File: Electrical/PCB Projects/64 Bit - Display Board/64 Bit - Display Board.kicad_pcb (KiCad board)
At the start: 4 copper layers, 200 x 75.1 mm, 60 parts, among them J1 Conn_01x03, J2 Conn_01x03, P1 610110249121, P2 610110249121, P3 610110249121, T1 IN-12A, T10 IN-12A, T2 IN-12A, T5 IN-12A, T6 IN-12A, T9 IN-12A, U1 TPIC6B595, U2 TPIC6B595, U3 TPIC6B595, U4 TPIC6B595, U5 TPIC6B595, U6 TPIC6B595, U7 TPIC6B595, U8 TPIC6B595

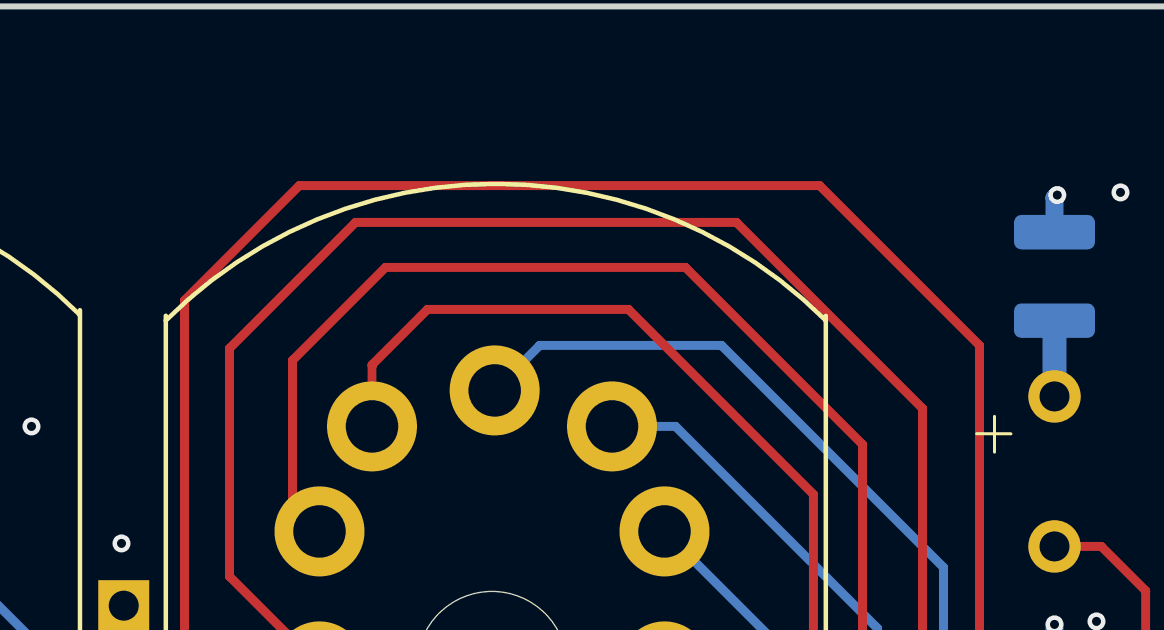
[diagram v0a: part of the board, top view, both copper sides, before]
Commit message: slight changes
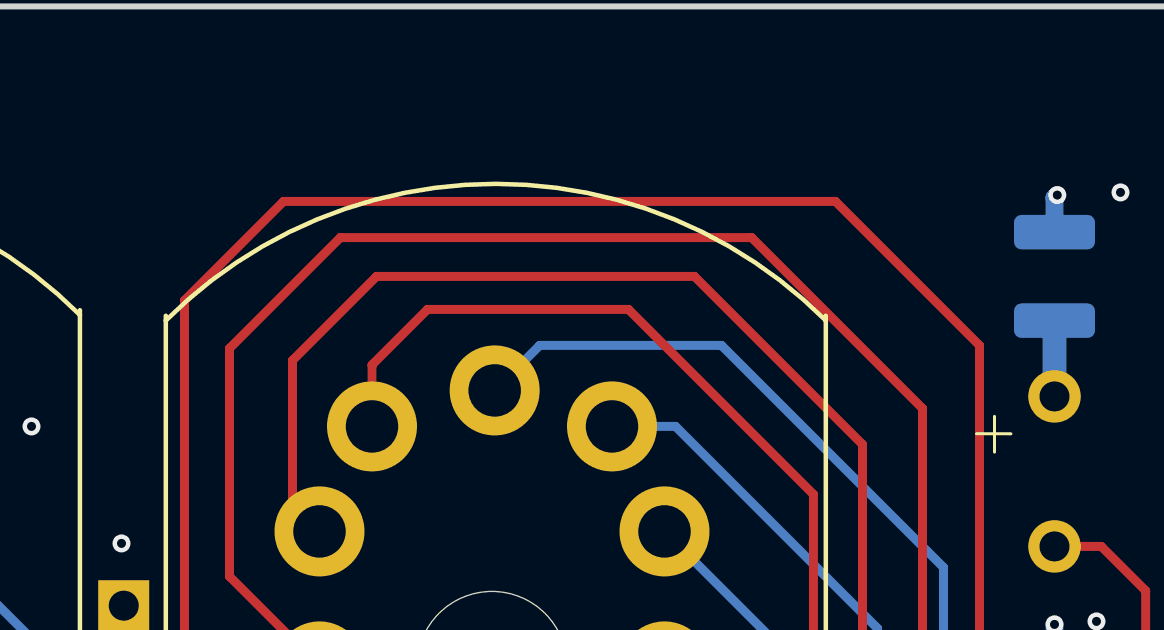
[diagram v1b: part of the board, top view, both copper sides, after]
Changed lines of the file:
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@@
+	)
+	(segment
+		(start 106.5 56.5)
+		(end 95.9 56.5)
+		(width 0.3)
+		(layer "F.Cu")
+		(net 72)
+	)
+	(segment
+		(start 93.1 59.3)
+		(end 93.1 64.1)
+		(width 0.3)
+		(layer "F.Cu")
+		(net 72)
+	)
+	(segment
+		(start 117.5 96.1)
+		(end 112.1 90.7)
+		(width 0.3)
+		(layer "F.Cu")
+		(net 72)
+	)
+	(segment
+		(start 112.1 62.1)
+		(end 106.5 56.5)
+		(width 0.3)
+		(layer "F.Cu")
+		(net 72)
+	)
+	(segment
+		(start 112.1 90.7)
+		(end 112.1 62.1)
+		(width 0.3)
+		(layer "F.Cu")
+		(net 72)
+	)
+	(segment
+		(start 121.567267 92.442808)
+		(end 121.567267 92.432733)
+		(width 0.3)
+		(layer "F.Cu")
+		(net 72)
 	)
 	(segment
@@
 	)
 	(segment
-		(start 117.5 96.1)
-		(end 112.1 90.7)
-		(width 0.3)
-		(layer "F.Cu")
-		(net 72)
-	)
-	(segment
-		(start 93.1 59.3)
-		(end 93.1 64.1)
-		(width 0.3)
-		(layer "F.Cu")
-		(net 72)
-	)
-	(segment
-		(start 112.1 62.1)
-		(end 106.2 56.2)
-		(width 0.3)
-		(layer "F.Cu")
-		(net 72)
-	)
-	(segment
-		(start 96.2 56.2)
+		(start 95.9 56.5)
 		(end 93.1 59.3)
-		(width 0.3)
-		(layer "F.Cu")
-		(net 72)
-	)
-	(segment
-		(start 121.567267 92.442808)
-		(end 121.567267 92.432733)
-		(width 0.3)
-		(layer "F.Cu")
-		(net 72)
-	)
-	(segment
-		(start 112.1 90.7)
-		(end 112.1 62.1)
-		(width 0.3)
-		(layer "F.Cu")
-		(net 72)
-	)
-	(segment
-		(start 106.2 56.2)
-		(end 96.2 56.2)
 		(width 0.3)
 		(layer "F.Cu")
@@
 	)
 	(segment
+		(start 91 58.9)
+		(end 91 66.5)
+		(width 0.3)
+		(layer "F.Cu")
+		(net 79)
+	)
+	(segment
+		(start 114.1 90.5)
+		(end 114.1 60.9)
+		(width 0.3)
+		(layer "F.Cu")
+		(net 79)
+	)
+	(segment
 		(start 91 66.5)
 		(end 94 69.5)
@@
 	)
 	(segment
+		(start 108.40569 55.20569)
+		(end 94.69431 55.20569)
+		(width 0.3)
+		(layer "F.Cu")
+		(net 79)
+	)
+	(segment
+		(start 114.1 60.9)
+		(end 108.40569 55.20569)
+		(width 0.3)
+		(layer "F.Cu")
+		(net 79)
+	)
+	(segment
 		(start 119.4 95.8)
 		(end 114.1 90.5)
@@
 	)
 	(segment
-		(start 107.9 54.7)
-		(end 95.2 54.7)
-		(width 0.3)
-		(layer "F.Cu")
-		(net 79)
-	)
-	(segment
-		(start 95.2 54.7)
-		(end 91 58.9)
-		(width 0.3)
-		(layer "F.Cu")
-		(net 79)
-	)
-	(segment
-		(start 91 58.9)
-		(end 91 66.5)
-		(width 0.3)
-		(layer "F.Cu")
-		(net 79)
-	)
-	(segment
 		(start 122.559167 93.340833)
 		(end 124 91.9)
@@
 	)
 	(segment
-		(start 114.1 90.5)
-		(end 114.1 60.9)
-		(width 0.3)
-		(layer "F.Cu")
-		(net 79)
-	)
-	(segment
-		(start 114.1 60.9)
-		(end 107.9 54.7)
+		(start 94.69431 55.20569)
+		(end 91 58.9)
 		(width 0.3)
 		(layer "F.Cu")
@@
 	)
 	(segment
+		(start 116 90.2)
+		(end 116 58.8)
+		(width 0.3)
+		(layer "F.Cu")
+		(net 80)
+	)
+	(segment
 		(start 120.811072 95.011072)
 		(end 116 90.2)
@@
 	)
 	(segment
-		(start 93.328049 53.471951)
+		(start 116 58.8)
+		(end 111.2 54)
+		(width 0.3)
+		(layer "F.Cu")
+		(net 80)
+	)
+	(segment
+		(start 111.2 54)
+		(end 92.8 54)
+		(width 0.3)
+		(layer "F.Cu")
+		(net 80)
+	)
+	(segment
+		(start 92.8 54)
 		(end 89.5 57.3)
 		(width 0.3)
@@
 	)
 	(segment
-		(start 110.671951 53.471951)
-		(end 93.328049 53.471951)
+		(start 89.5 69.5)
+		(end 94 74)
+		(width 0.3)
+		(layer "F.Cu")
+		(net 80)
+	)
+	(segment
+		(start 89.5 57.3)
+		(end 89.5 69.5)
 		(width 0.3)
 		(layer "F.Cu")
@@
 	)
 	(segment
-		(start 89.5 69.5)
-		(end 94 74)
-		(width 0.3)
-		(layer "F.Cu")
-		(net 80)
-	)
-	(segment
 		(start 122.591105 95.011072)
 		(end 120.811072 95.011072)
-		(width 0.3)
-		(layer "F.Cu")
-		(net 80)
-	)
-	(segment
-		(start 89.5 57.3)
-		(end 89.5 69.5)
-		(width 0.3)
-		(layer "F.Cu")
-		(net 80)
-	)
-	(segment
-		(start 116 90.2)
-		(end 116 58.8)
-		(width 0.3)
-		(layer "F.Cu")
-		(net 80)
-	)
-	(segment
-		(start 116 58.8)
-		(end 110.671951 53.471951)
 		(width 0.3)
 		(layer "F.Cu")
@@
 		(net 2)
 		(net_name "GND")
-		(layers "F.Cu" "B.Cu")
+		(layers "F.Cu" "B.Cu" "In1.Cu")
 		(hatch edge 0.5)
 		(priority 1)
@@
 		(net 2)
 		(net_name "GND")
-		(layers "F.Cu" "B.Cu")
+		(layers "F.Cu" "B.Cu" "In1.Cu")
 		(hatch edge 0.5)
 		(priority 1)
@@
 		(net 2)
 		(net_name "GND")
-		(layers "F.Cu" "B.Cu")
+		(layers "F.Cu" "B.Cu" "In1.Cu")
 		(hatch edge 0.5)
 		(priority 1)
@@
 		(net 2)
 		(net_name "GND")
-		(layers "F.Cu" "B.Cu")
+		(layers "F.Cu" "B.Cu" "In1.Cu")
 		(hatch edge 0.5)
 		(priority 1)
@@
 		(net 2)
 		(net_name "GND")
-		(layers "F.Cu" "B.Cu")
+		(layers "F.Cu" "B.Cu" "In1.Cu")
 		(hatch edge 0.5)
 		(priority 1)
